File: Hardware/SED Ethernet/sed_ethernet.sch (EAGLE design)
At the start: 30 parts, among them IC1 ENC28J60SSOP, Q2 25MHz

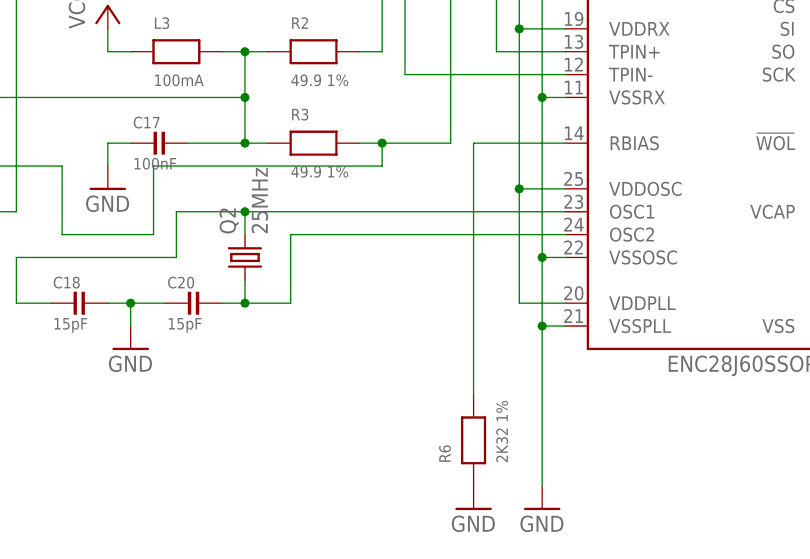
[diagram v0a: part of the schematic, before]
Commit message: Cristal con toma de tierra
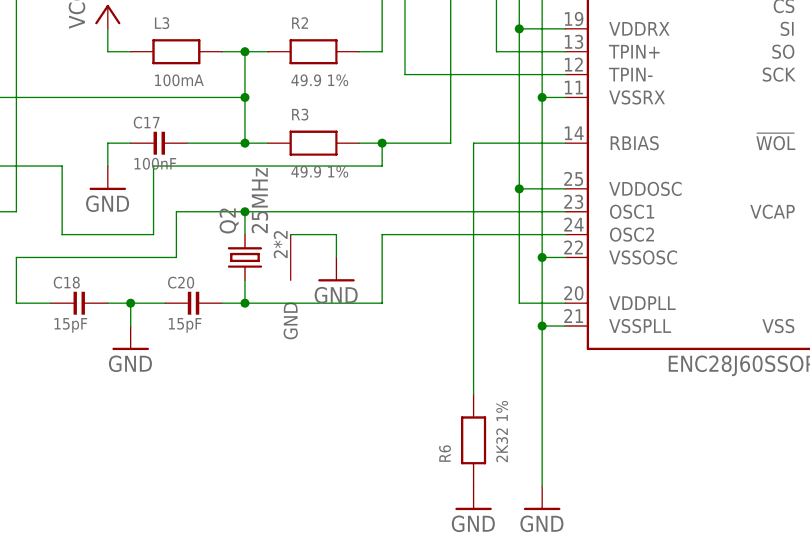
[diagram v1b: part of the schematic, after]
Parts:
- Q2: device SparkFun:CRYSTAL5X3 -> sed_library:CRYSTAL5X3
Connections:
- net GND: now also Q2.GND
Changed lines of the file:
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@@
 <part name="GND6" library="supply1" deviceset="GND" device=""/>
 <part name="GND8" library="supply1" deviceset="GND" device=""/>
-<part name="Q2" library="SparkFun" deviceset="CRYSTAL" device="5X3" value="25MHz"/>
+<part name="Q2" library="sed_library" deviceset="CRYSTAL" device="5X3" value="25MHz"/>
 <part name="GND7" library="supply1" deviceset="GND" device=""/>
 <part name="GND9" library="supply1" deviceset="GND" device=""/>
@@
 <part name="L3" library="hackermesh" deviceset="RESISTENCIA-0805" device="" value="100mA"/>
 <part name="C21" library="hackermesh" deviceset="CONDENSADOR-0805" device="" value="10uF low esr (&lt;5ohm)"/>
+<part name="GND12" library="supply1" deviceset="GND" device=""/>
 </parts>
 <sheets>
@@
 <instance part="L3" gate="&gt;NAME" x="167.64" y="40.64"/>
 <instance part="C21" gate="G$1" x="251.46" y="8.89" rot="R90"/>
+<instance part="GND12" gate="1" x="185.42" y="15.24"/>
 </instances>
 <busses>
@@
 <pinref part="GND10" gate="1" pin="GND"/>
 <pinref part="R6" gate="&gt;NAME" pin="1"/>
+</segment>
+<segment>
+<pinref part="Q2" gate="G$1" pin="GND"/>
+<pinref part="GND12" gate="1" pin="GND"/>
+<wire x1="180.34" y1="20.32" x2="185.42" y2="20.32" width="0.1524" layer="91"/>
+<wire x1="185.42" y1="20.32" x2="185.42" y2="17.78" width="0.1524" layer="91"/>
 </segment>
 </net>
@@
 <pinref part="Q2" gate="G$1" pin="1"/>
 <pinref part="IC1" gate="G$1" pin="OSC2"/>
-<wire x1="210.82" y1="20.32" x2="180.34" y2="20.32" width="0.1524" layer="91"/>
-<wire x1="180.34" y1="20.32" x2="180.34" y2="12.7" width="0.1524" layer="91"/>
-<wire x1="180.34" y1="12.7" x2="175.26" y2="12.7" width="0.1524" layer="91"/>
+<wire x1="210.82" y1="20.32" x2="190.5" y2="20.32" width="0.1524" layer="91"/>
+<wire x1="190.5" y1="20.32" x2="190.5" y2="12.7" width="0.1524" layer="91"/>
 <pinref part="C20" gate="G$1" pin="2"/>
-</segment>
-</net>
+<wire x1="190.5" y1="12.7" x2="175.26" y2="12.7" width="0.1524" layer="91"/>
+</segment>
+</net>
